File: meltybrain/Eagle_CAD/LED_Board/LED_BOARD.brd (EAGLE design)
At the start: 56 x 12 mm, 17 parts, among them J1 SM04B-SRSS-TB(LF)(SN), U1 DOTSTAR, U2 DOTSTAR, U3 DOTSTAR, U4 DOTSTAR, U5 DOTSTAR, U6 DOTSTAR, U7 DOTSTAR, U8 DOTSTAR

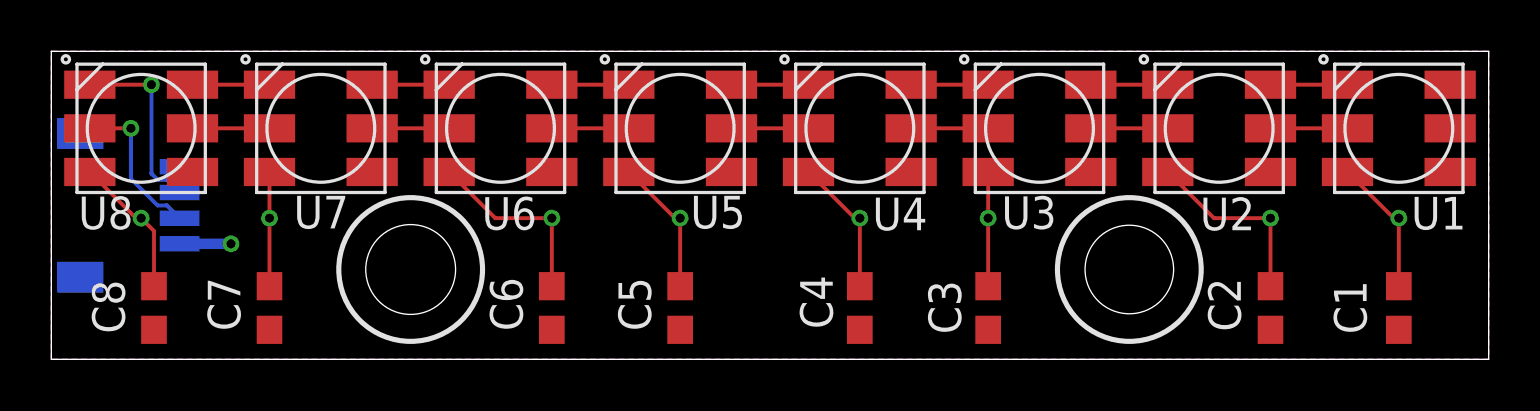
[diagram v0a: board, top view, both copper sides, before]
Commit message: led board cad
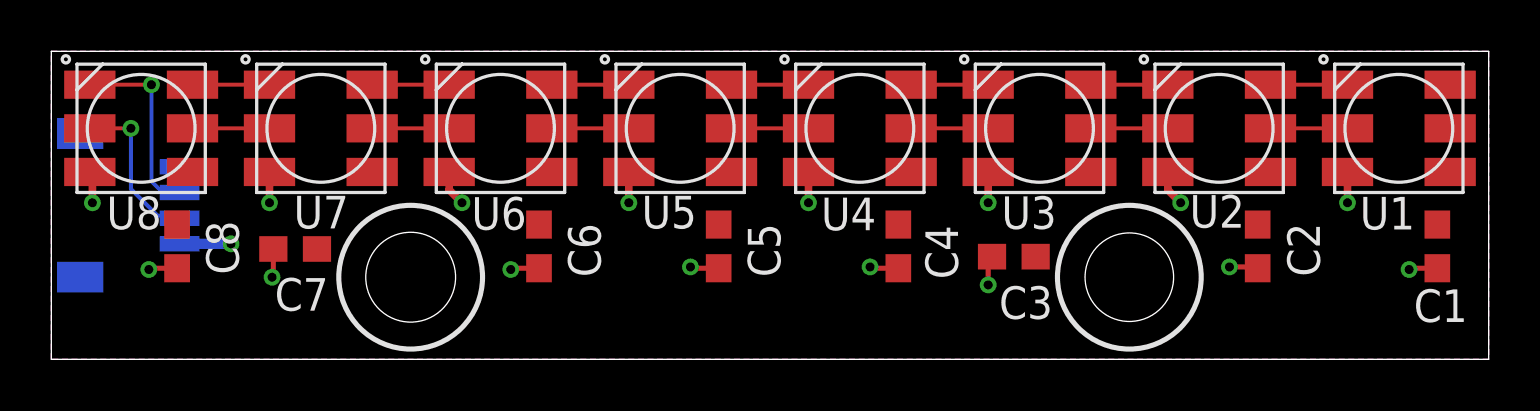
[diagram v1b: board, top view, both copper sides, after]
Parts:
- moved C1 2.83 mm to (54.0, 4.40), turned to 270 degrees
- moved C4 2.83 mm to (33.0, 4.40), turned to 270 degrees
- moved C5 2.83 mm to (26.0, 4.40), turned to 270 degrees
- moved C8 2.56 mm to (4.90, 4.40), turned to 270 degrees
- moved C7 2.51 mm to (9.50, 4.30), turned to 180 degrees
- moved C2 2.45 mm to (47.0, 4.40), turned to 270 degrees
- moved C6 2.45 mm to (19.0, 4.40), turned to 270 degrees
- moved C3 2.24 mm to (37.5, 4.00), turned to 180 degrees
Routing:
- net GND: track 45.5 -> 19.1 mm, vias 8 -> 16
